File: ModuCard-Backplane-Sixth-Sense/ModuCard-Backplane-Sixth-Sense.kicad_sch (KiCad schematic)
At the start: 14 parts

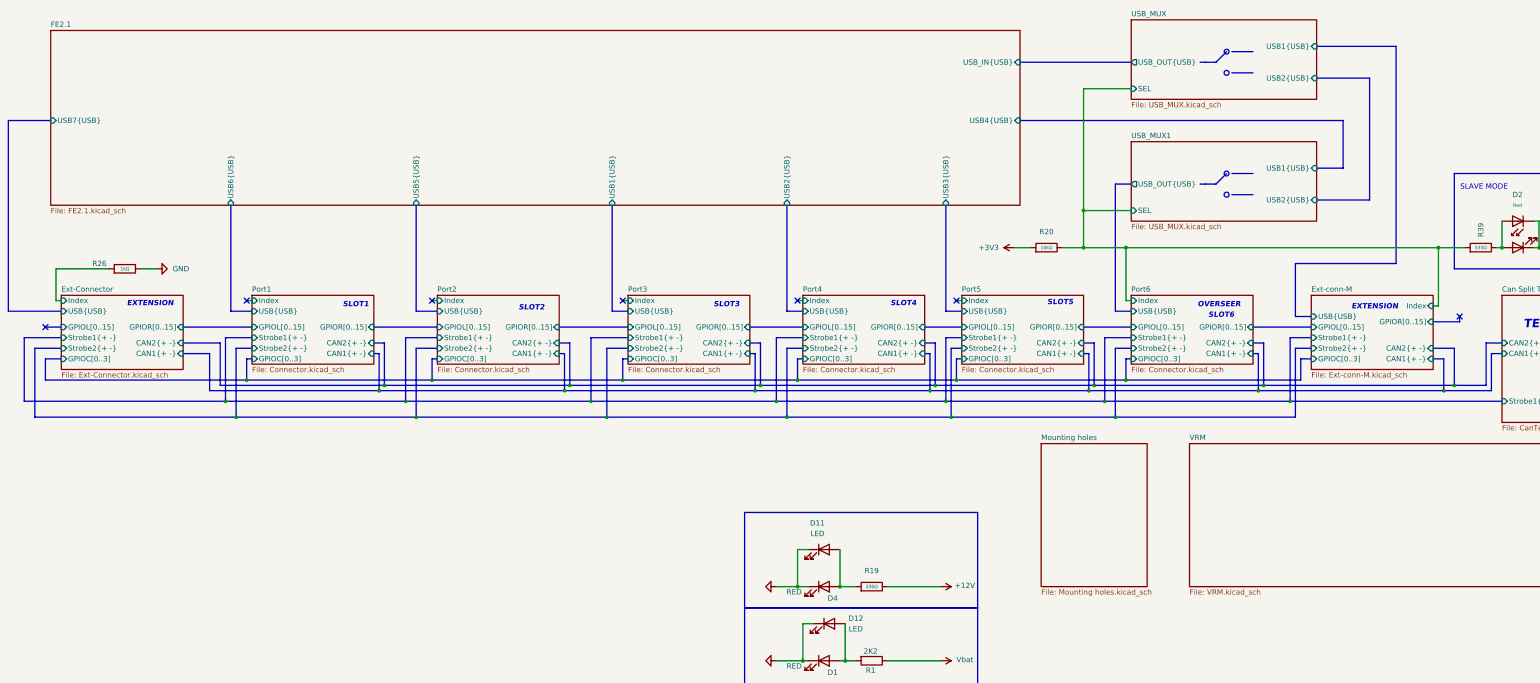
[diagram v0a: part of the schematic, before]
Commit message: project overhaul
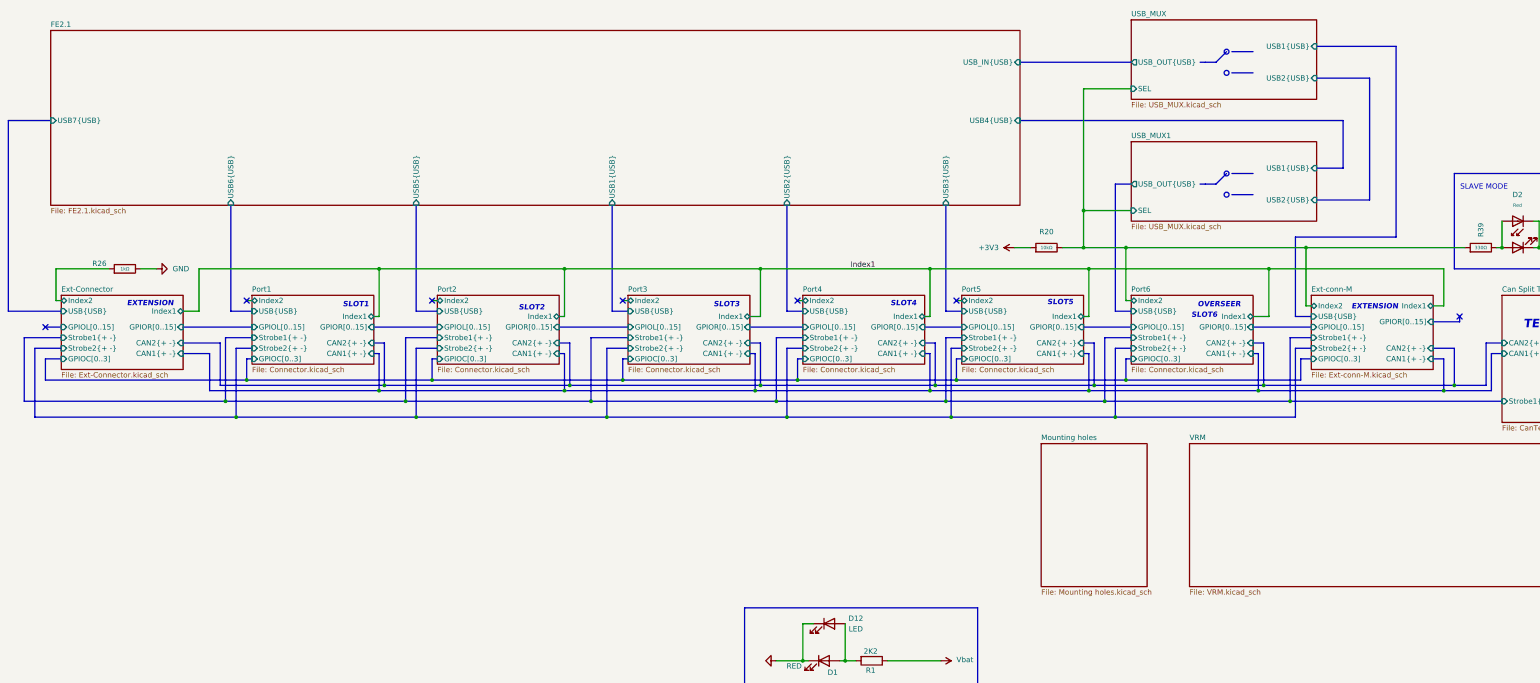
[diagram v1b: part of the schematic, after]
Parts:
- removed D11: LED, LED_THT:LED_D3.0mm, symbol Device:LED
- removed D4: RED, Diode_SMD:D_0402_1005Metric, symbol Device:LED
- removed R19: 330Ω, PCM_JLCPCB:R_0402, symbol PCM_JLCPCB-Resistors:0402,330Ω
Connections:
- net Ext-Connector/Index renamed Ext-Connector/Index2
- net Ext-conn-M/Index renamed Ext-conn-M/Index2
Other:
- sheet Ext-Connector ports: added Index1, Index2; removed Index
- sheet Ext-conn-M ports: added Index1, Index2; removed Index
- sheet Port1 ports: added Index1, Index2; removed Index
- sheet Port2 ports: added Index1, Index2; removed Index
- sheet Port3 ports: added Index1, Index2; removed Index
- sheet Port4 ports: added Index1, Index2; removed Index
- sheet Port5 ports: added Index1, Index2; removed Index
- sheet Port6 ports: added Index1, Index2; removed Index

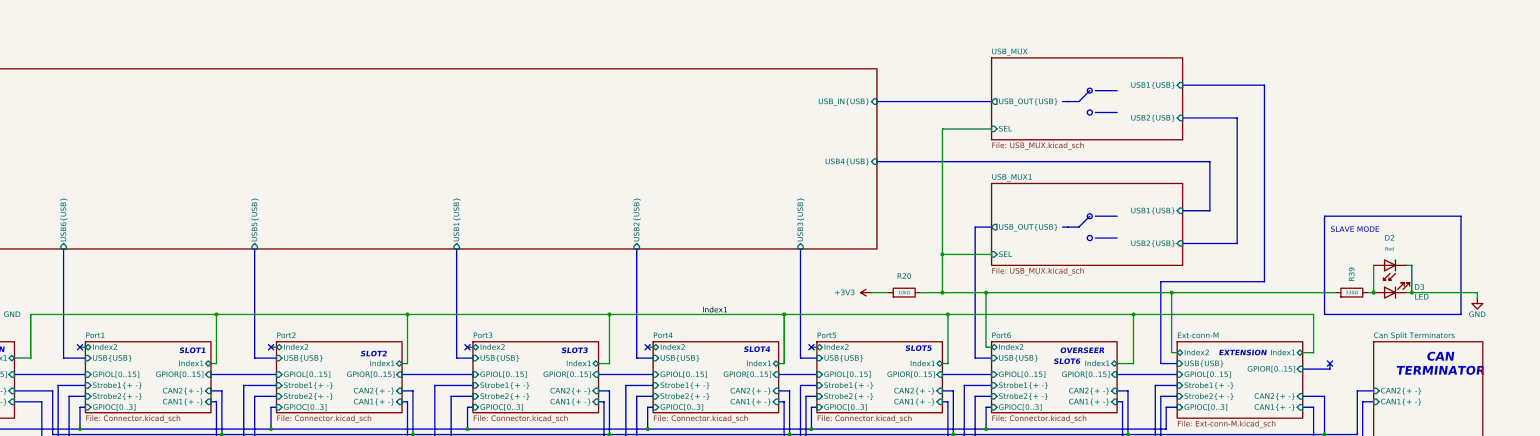
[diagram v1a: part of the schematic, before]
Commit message: final check pinout
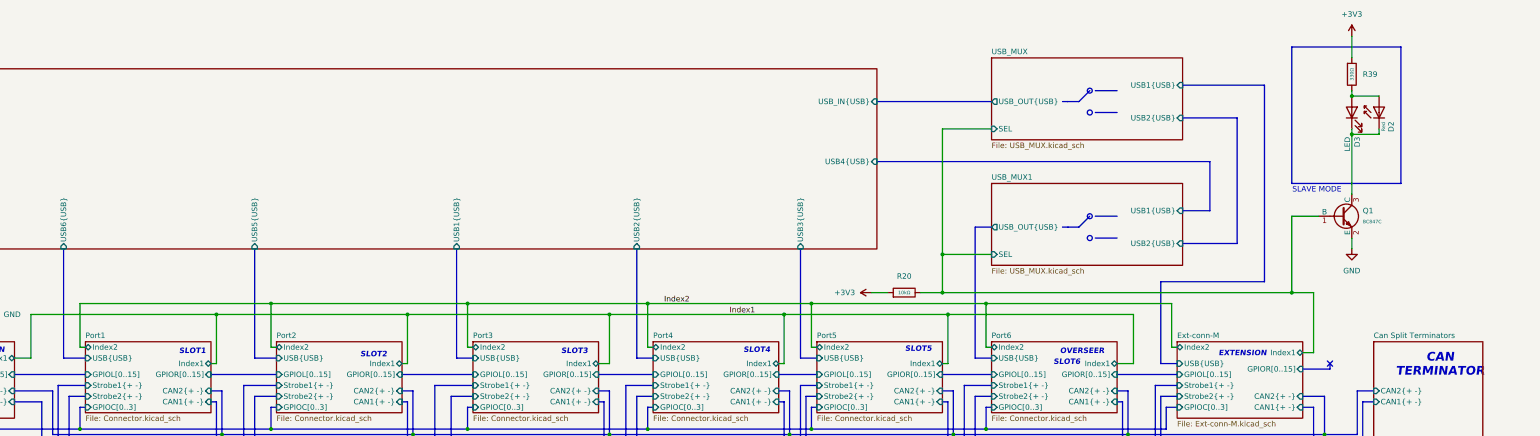
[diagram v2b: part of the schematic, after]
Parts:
- added Q1: BC847C, PCM_JLCPCB:Q_SOT-23, symbol PCM_JLCPCB-Transistors:NPN,BC847C
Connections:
- net +3V3: now also R39.1
- net GND: now also Q1.2 (E); no longer D2.1, D3.1 (K)
- net Ext-conn-M/Index2 renamed Ext-conn-M/Index1
- net Ext-conn-M/Index1: now also Q1.1 (B); no longer R39.1
- new net: D2.1, D3.1 (K), Q1.3 (C)
- no-connect marks 7 -> 2
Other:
- moved on the sheet: D2, D3, R39

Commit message: fin
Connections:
- net Ext-Connector/Index2 renamed Ext-Connector/Index1
- no-connect marks 2 -> 8
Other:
- moved on the sheet: D1, D12, D13, D8, R1, R18, R26
